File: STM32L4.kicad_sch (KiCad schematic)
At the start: 32 parts, among them J1 Conn_01x04_Pin, U11 MR20H40, U12 TCAN334, U20 STM32L476RGTx, Y1 8 MHZ Oscillator

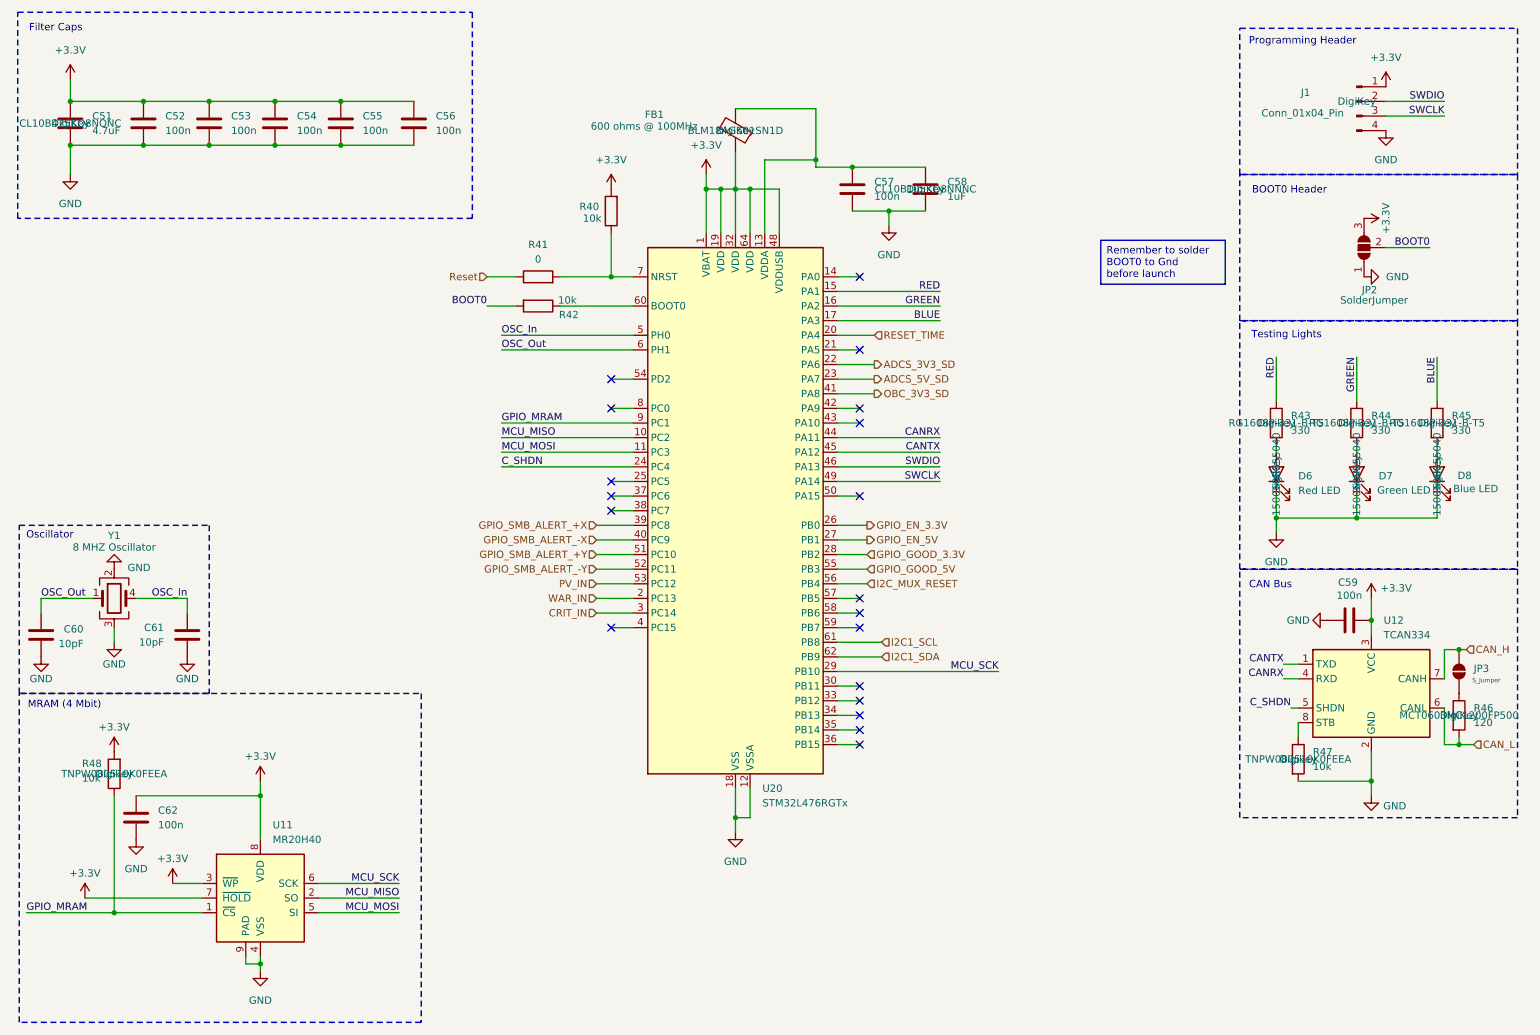
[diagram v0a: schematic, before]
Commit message: A bunch of misc schematic changes
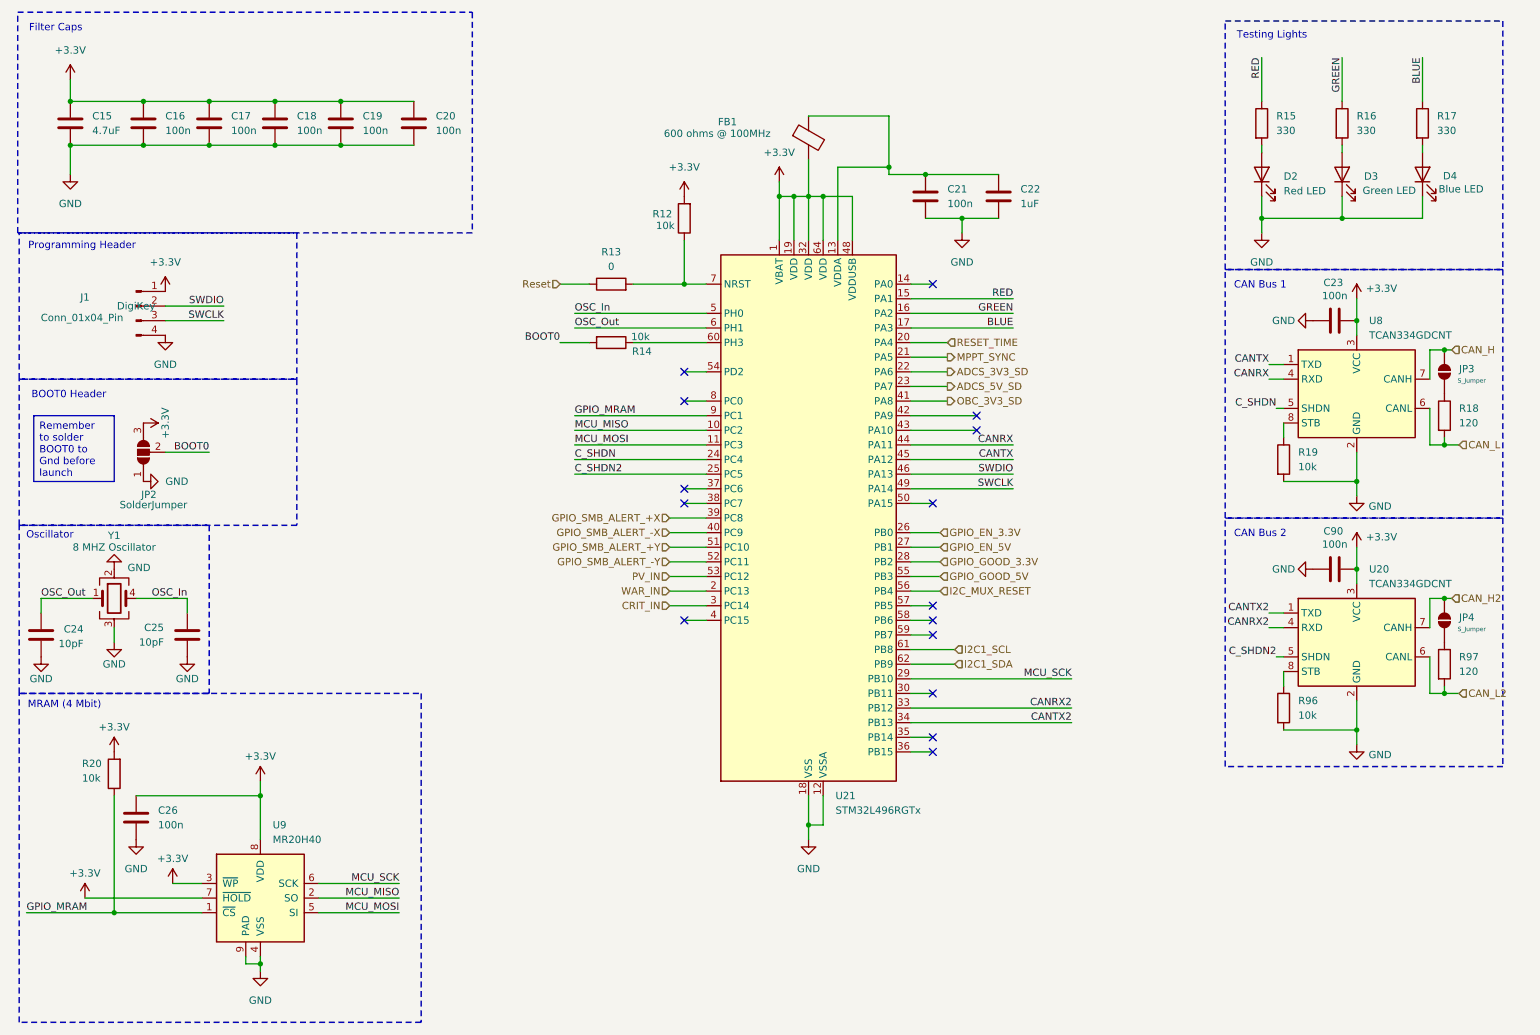
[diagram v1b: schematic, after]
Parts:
- removed U20: STM32L476RGTx, Package_QFP:LQFP-64_10x10mm_P0.5mm, symbol MCU_ST_STM32L4:STM32L476RGTx
- added C90: 100n, Capacitor_SMD:C_0603_1608Metric, symbol Device:C
- added JP4: S_Jumper, Jumper:SolderJumper-2_P1.3mm_Open_TrianglePad1.0x1.5mm, symbol Jumper:SolderJumper_2_Open
- added R96: 10k, Resistor_SMD:R_0805_2012Metric, symbol Device:R
- added R97: 120, Resistor_SMD:R_0603_1608Metric, symbol Device:R
- added U20: TCAN334GDCNT, Package_TO_SOT_SMD:SOT-23-8, symbol Interface_CAN_LIN:TCAN334
- added U21: STM32L496RGTx, Package_QFP:LQFP-64_10x10mm_P0.5mm, symbol MCU_ST_STM32L4:STM32L496RGTx
- U8: renamed from U12; value TCAN334 -> TCAN334GDCNT; footprint Package_SO:SOIC-8_3.9x4.9mm_P1.27mm -> Package_TO_SOT_SMD:SOT-23-8
- renumbered C51 to C15, C52 to C16, C53 to C17, C54 to C18, C55 to C19, C56 to C20, C57 to C21, C58 to C22, C59 to C23, C60 to C24, C61 to C25, C62 to C26, D6 to D2, D7 to D3, D8 to D4, R40 to R12, R41 to R13, R42 to R14, R43 to R15, R44 to R16, R45 to R17, R46 to R18, R47 to R19, R48 to R20, U11 to U9
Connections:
- net +3.3V: now also C90.2, U20.3 (VCC), U21.1 (VBAT), U21.19 (VDD), U21.32 (VDD), U21.48 (VDDUSB), U21.64 (VDD)
- net ADCS_3V3_SD: now also U21.22 (PA6)
- net ADCS_5V_SD: now also U21.23 (PA7)
- net BLUE: now also U21.17 (PA3)
- net CANRX: now also U21.44 (PA11)
- net CANTX: now also U21.45 (PA12)
- net CRIT_IN: now also U21.3 (PC14)
- net C_SHDN: now also U21.24 (PC4)
- net GND: now also C90.1, R96.2, U20.2 (GND), U21.12 (VSSA), U21.18 (VSS), U21.31 (VSS), U21.47 (VSS), U21.63 (VSS)
- net GPIO_EN_3.3V: now also U21.26 (PB0)
- net GPIO_EN_5V: now also U21.27 (PB1)
- net GPIO_GOOD_3.3V: now also U21.28 (PB2)
- net GPIO_GOOD_5V: now also U21.55 (PB3)
- net GPIO_MRAM: now also U21.9 (PC1)
- net GPIO_SMB_ALERT_+X: now also U21.39 (PC8)
- net GPIO_SMB_ALERT_+Y: now also U21.51 (PC10)
- net GPIO_SMB_ALERT_-X: now also U21.40 (PC9)
- net GPIO_SMB_ALERT_-Y: now also U21.52 (PC11)
- net GREEN: now also U21.16 (PA2)
- net I2C1_SCL: now also U21.61 (PB8)
- net I2C1_SDA: now also U21.62 (PB9)
- net I2C_MUX_RESET: now also U21.56 (PB4)
- net MCU_MISO: now also U21.10 (PC2)
- net MCU_MOSI: now also U21.11 (PC3)
- net MCU_SCK: now also U21.29 (PB10)
- net OBC_3V3_SD: now also U21.41 (PA8)
- net OSC_In: now also U21.5 (PH0)
- net OSC_Out: now also U21.6 (PH1)
- net PV_IN: now also U21.53 (PC12)
- net RED: now also U21.15 (PA1)
- net RESET_TIME: now also U21.20 (PA4)
- net SWCLK: now also U21.49 (PA14)
- net SWDIO: now also U21.46 (PA13)
- net WAR_IN: now also U21.2 (PC13)
- net at R12.1, R13.2: now also U21.7 (NRST)
- net at C21.1, C22.1, FB1.1: now also U21.13 (VDDA)
- net at R14.1: now also U21.60 (PH3)
- new net: JP4.1 (A), R97.1
- new net: R96.1, U20.8 (STB)
- new net CANRX2: U20.4 (RXD), U21.33 (PB12)
- new net CANTX2: U20.1 (TXD), U21.34 (PB13)
- new net CAN_H2: JP4.2 (B), U20.7 (CANH)
- new net CAN_L2: R97.2, U20.6 (CANL)
- new net C_SHDN2: U20.5 (SHDN), U21.25 (PC5)
- new net MPPT_SYNC: U21.21 (PA5)
- no-connect marks 19 -> 15
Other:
- note added: "CAN Bus 1"
- note added: "CAN Bus 2"
- note removed: "CAN Bus"
- moved on the sheet: C21, C22, C23, D2, D3, D4, FB1, J1, JP2, JP3, R12, R13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
